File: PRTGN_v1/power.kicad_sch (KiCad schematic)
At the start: 20 parts, among them IC1 TPS565242DRLR, J1 Barrel_Jack, J2 Screw_Terminal_01x02, J4 Screw_Terminal_01x02, Q1 Q_PMOS, Q2 Q_PMOS, SW1 SW_DPDT_x2

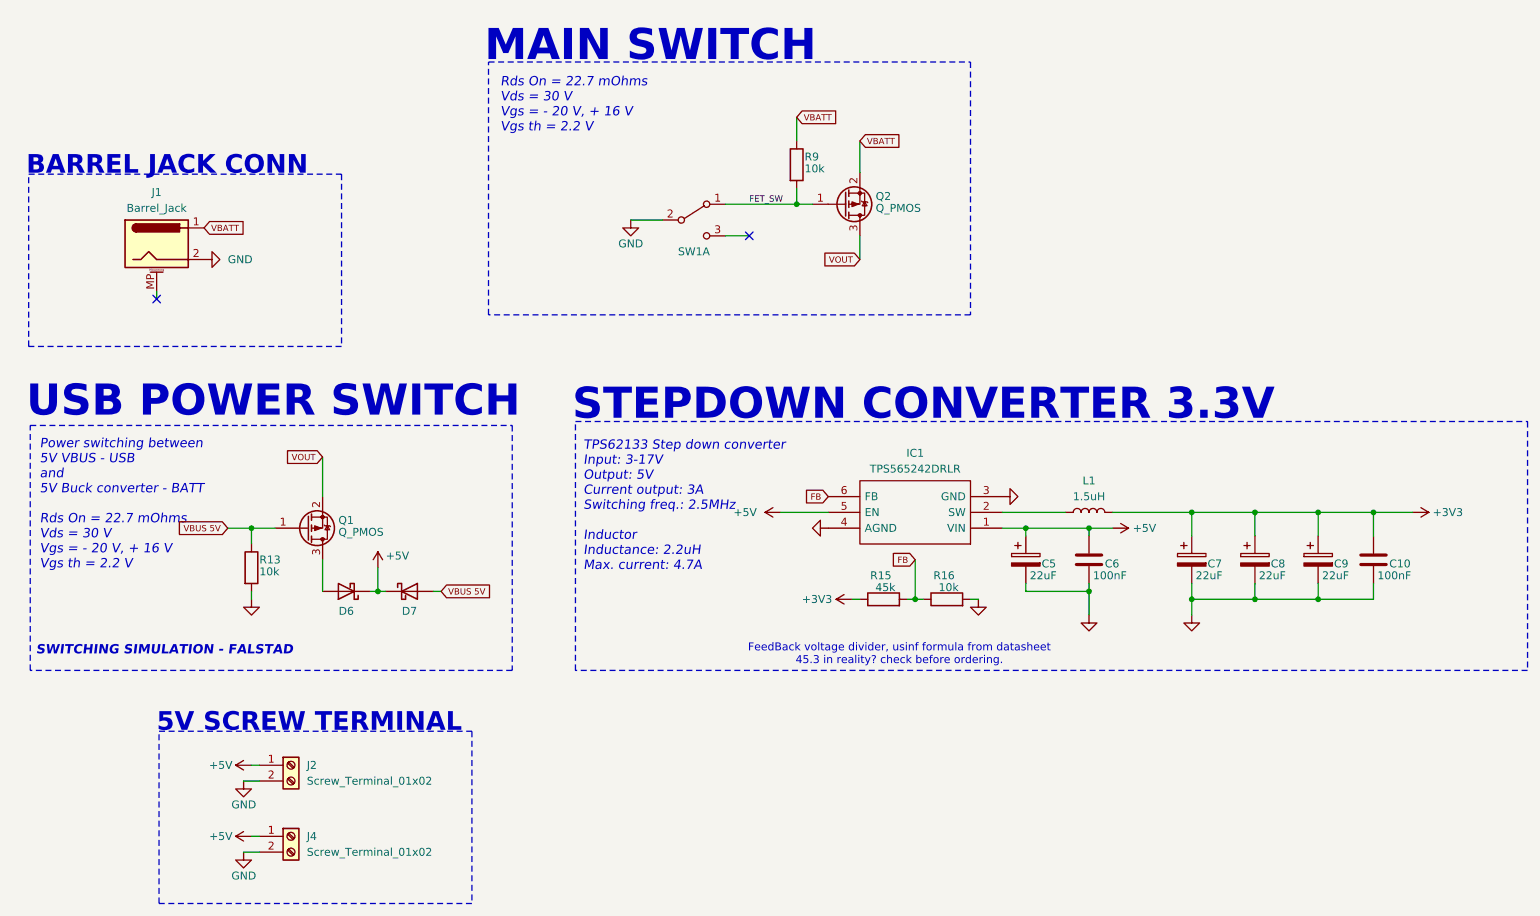
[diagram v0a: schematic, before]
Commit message: upd
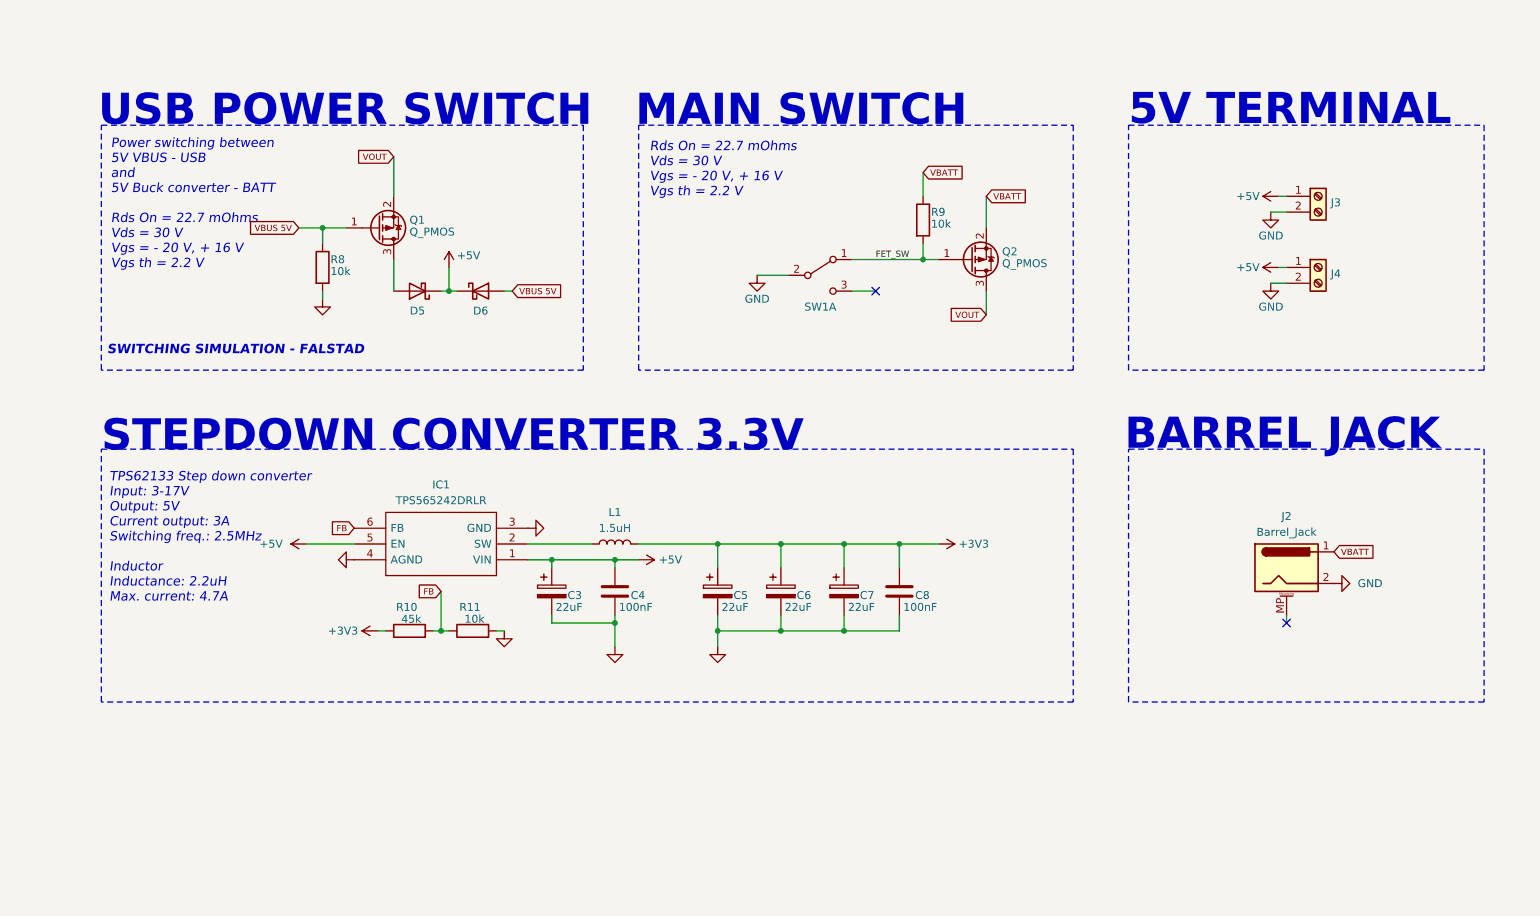
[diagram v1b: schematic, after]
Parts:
- renumbered C5 to C3, C6 to C4, C7 to C5, C8 to C6, C9 to C7, C10 to C8, D6 to D5, D7 to D6, J1 to J2, J2 to J3, R15 to R10, R16 to R11, R13 to R8
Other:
- note added: "5V TERMINAL"
- note added: "BARREL JACK"
- note removed: "5V SCREW TERMINAL"
- note removed: "BARREL JACK CONN"
- note removed: "FeedBack voltage divider, usinf formula from datasheet 45.3 in reality? check before ordering."
- moved on the sheet: C3, C4, C5, C6, C7, C8, D5, D6, IC1, J2, J3, J4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
